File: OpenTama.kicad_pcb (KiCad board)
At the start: 2 copper layers, 45 x 58.2 mm, 65 parts, among them J1 Conn_01x09, J2 Conn_01x14, J3 Conn_01x07, J4 USB_C_Receptacle_USB2.0, J5 Conn_01x14, Q1 BSS138, Q2 BSS138, Q3 BSS84, SW1 LEFT, SW2 MIDDLE, SW3 RIGHT, U1 TPS62203DBV, U2 LTC4054ES5-4.2, U3 STM32L072CBTx, U4 USBLC6-2SC6, Y1 32768Hz - 12,5 pF

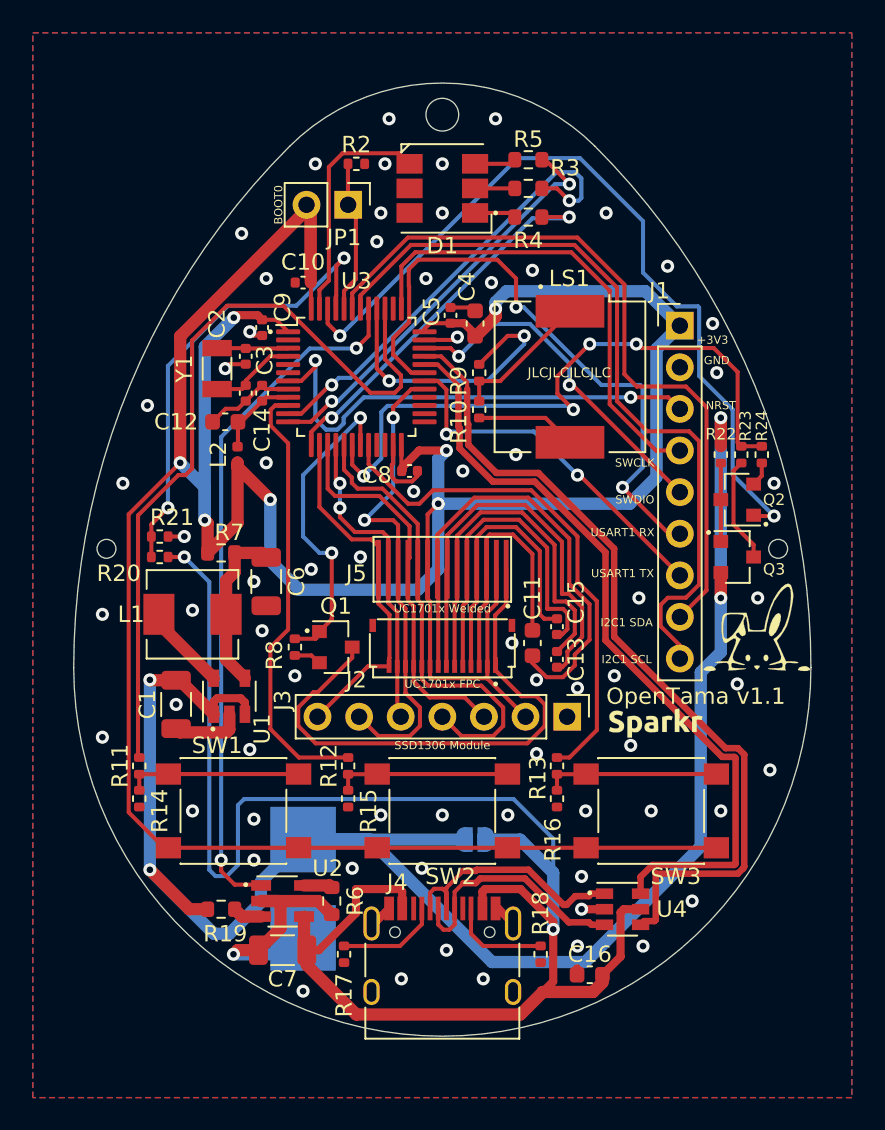
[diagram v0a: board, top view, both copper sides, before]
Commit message: PCB Trace, Via, Zone Reset
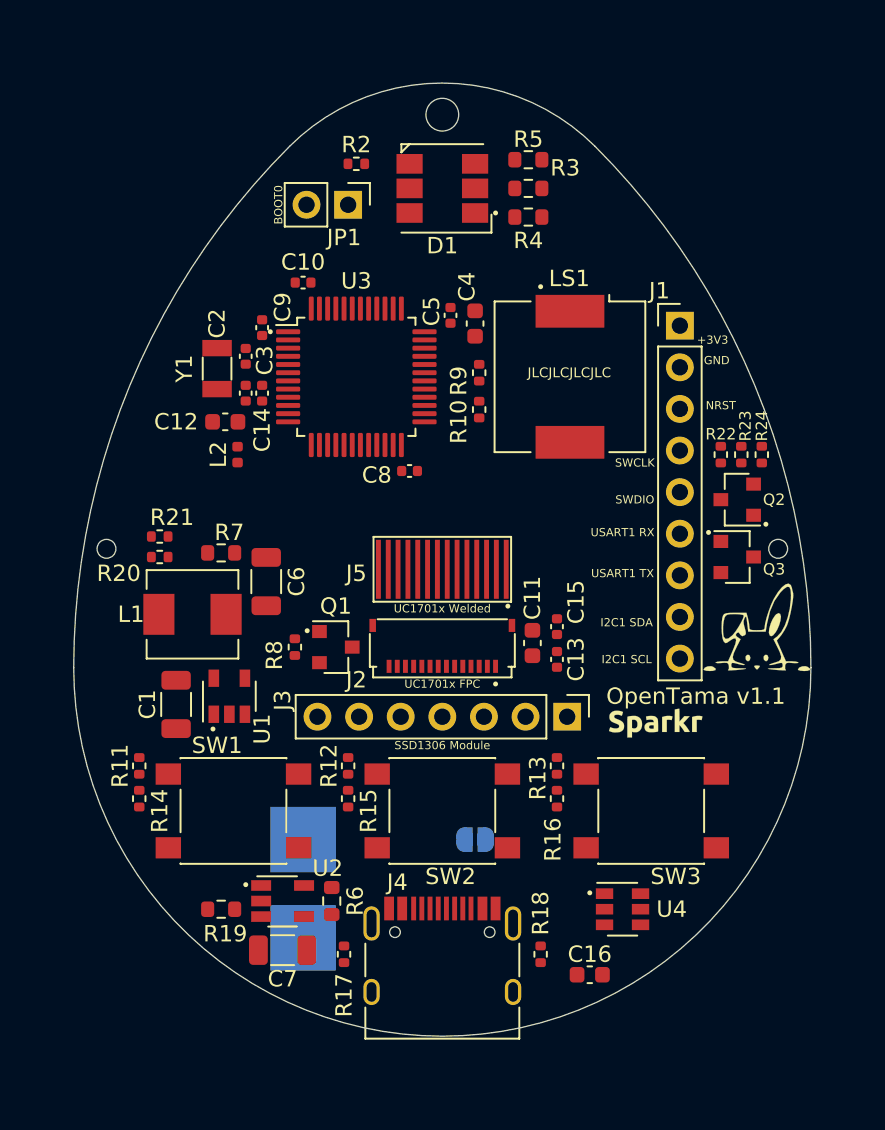
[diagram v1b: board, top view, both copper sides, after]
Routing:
- net +3V3: track 217.2 -> 0.00 mm, vias 7 -> 0
- net +BATT: track 108.7 -> 0.00 mm, vias 4 -> 0
- net +5V: track 106.7 -> 0.00 mm, vias 2 -> 0
- net -BATT: track 95.5 -> 0.00 mm, vias 69 -> 0
- net USB_D+: track 51.2 -> 0.00 mm
- net VBATT_MEAS: track 49.9 -> 0.00 mm, vias 2 -> 0
- net LEFT_BTN: track 48.3 -> 0.00 mm
- net USB_D-: track 47.9 -> 0.00 mm
- net I2C1_SCL: track 47.2 -> 0.00 mm
- net I2C1_SDA: track 45.0 -> 0.00 mm
- net NCHARG: track 42.5 -> 0.00 mm, vias 2 -> 0
- net VBATT_ANA: track 39.4 -> 0.00 mm, vias 4 -> 0
- net USART1_RX: track 38.0 -> 0.00 mm, vias 2 -> 0
- net Net-(J2-Pin_1): track 34.0 -> 0.00 mm
- net RIGHT_BTN: track 31.9 -> 0.00 mm
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- removed copper zone on B.Cu, net -BATT
- removed copper zone on F.Cu, net -BATT
